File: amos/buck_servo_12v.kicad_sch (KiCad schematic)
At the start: 42 parts, among them Q301 CSD18532Q5B, Q302 CSD18532Q5B, U301 LM5145RGYR

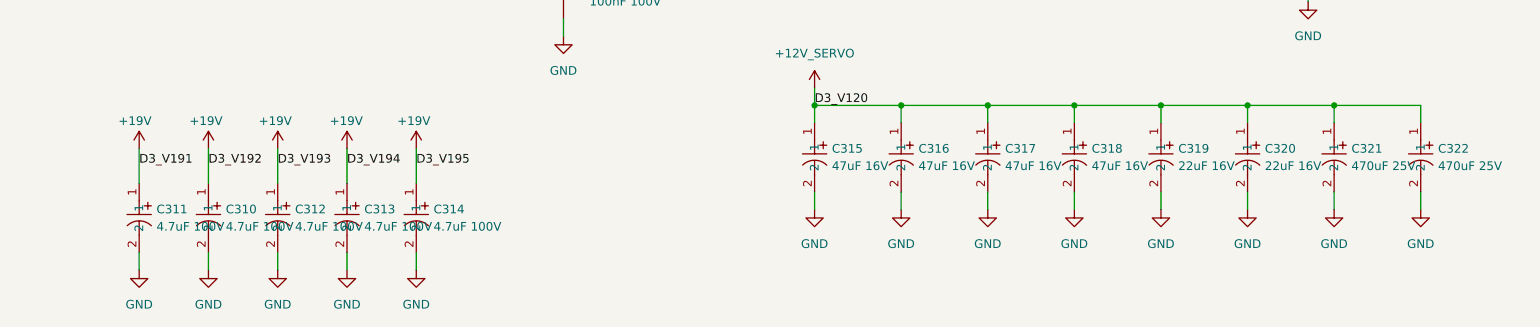
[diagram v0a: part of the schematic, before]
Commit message: update
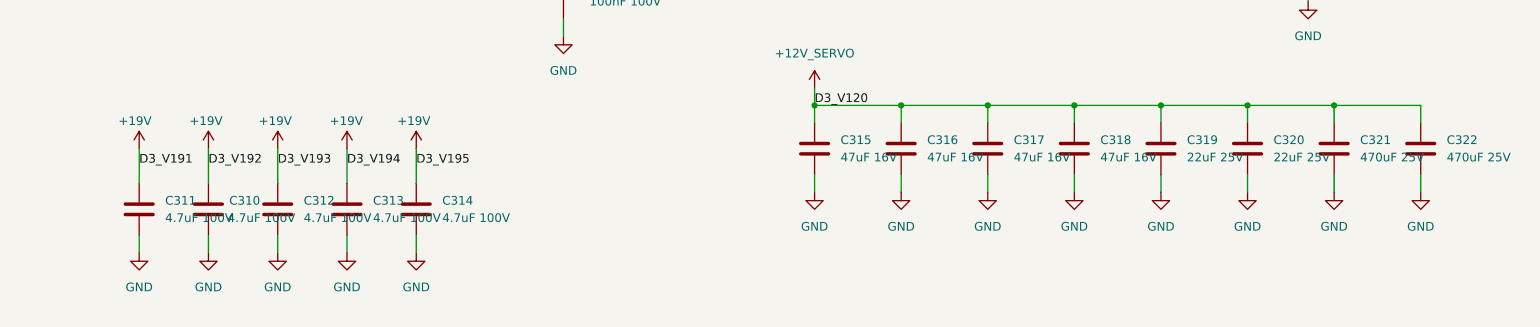
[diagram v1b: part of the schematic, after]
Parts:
- C309: footprint (none) -> Capacitor_SMD:C_0805_2012Metric; LCSC Part (none) -> C28233
- C310, C311, C312, C313, C314: footprint easyeda2kicad:CAP-SMD_BD10.0-L10.3-W10.3-LS11.3-FD -> Capacitor_SMD:C_1210_3225Metric; symbol easyeda2kicad:RVE470UF35V167RV084 -> Device:C; LCSC Part C5155332 -> C342614; MPN RVE470UF35V167RV084 -> (none); Manufacturer KNSCHA(科尼盛) -> (none)
- C315, C316, C317, C318: footprint easyeda2kicad:CAP-SMD_BD10.0-L10.3-W10.3-LS11.3-FD -> Capacitor_SMD:C_1210_3225Metric; symbol easyeda2kicad:RVE470UF35V167RV084 -> Device:C; LCSC Part C5155332 -> C77101; MPN RVE470UF35V167RV084 -> (none); Manufacturer KNSCHA(科尼盛) -> (none)
- C319, C320: value 22uF 16V -> 22uF 25V; footprint easyeda2kicad:CAP-SMD_BD10.0-L10.3-W10.3-LS11.3-FD -> Capacitor_SMD:C_1210_3225Metric; symbol easyeda2kicad:RVE470UF35V167RV084 -> Device:C; LCSC Part C5155332 -> C2918511; MPN RVE470UF35V167RV084 -> (none); Manufacturer KNSCHA(科尼盛) -> (none)
- C321, C322: footprint easyeda2kicad:CAP-SMD_BD10.0-L10.3-W10.3-LS11.3-FD -> easyeda2kicad:CAP-SMD_BD8.0-L8.3-W8.3-LS9.0-FD_H10.5; symbol easyeda2kicad:RVE470UF35V167RV084 -> Device:C; LCSC Part C5155332 -> C46550466; MPN RVE470UF35V167RV084 -> (none); Manufacturer KNSCHA(科尼盛) -> (none)
